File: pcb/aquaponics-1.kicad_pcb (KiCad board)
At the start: 2 copper layers, 67.3 x 63.5 mm, 17 parts, among them J1 5V Power Source, J2 Screw_Terminal_01x02, J3 Water Level Sensor, J4 Rain Sensor, J5 Conn_01x02_Female, M1 Growbed Pump, M2 Overflow Pump, M3 Fish Feeder, Q1 TIP120, Q2 TIP120, Q3 TIP120, U1 Arduino_Nano

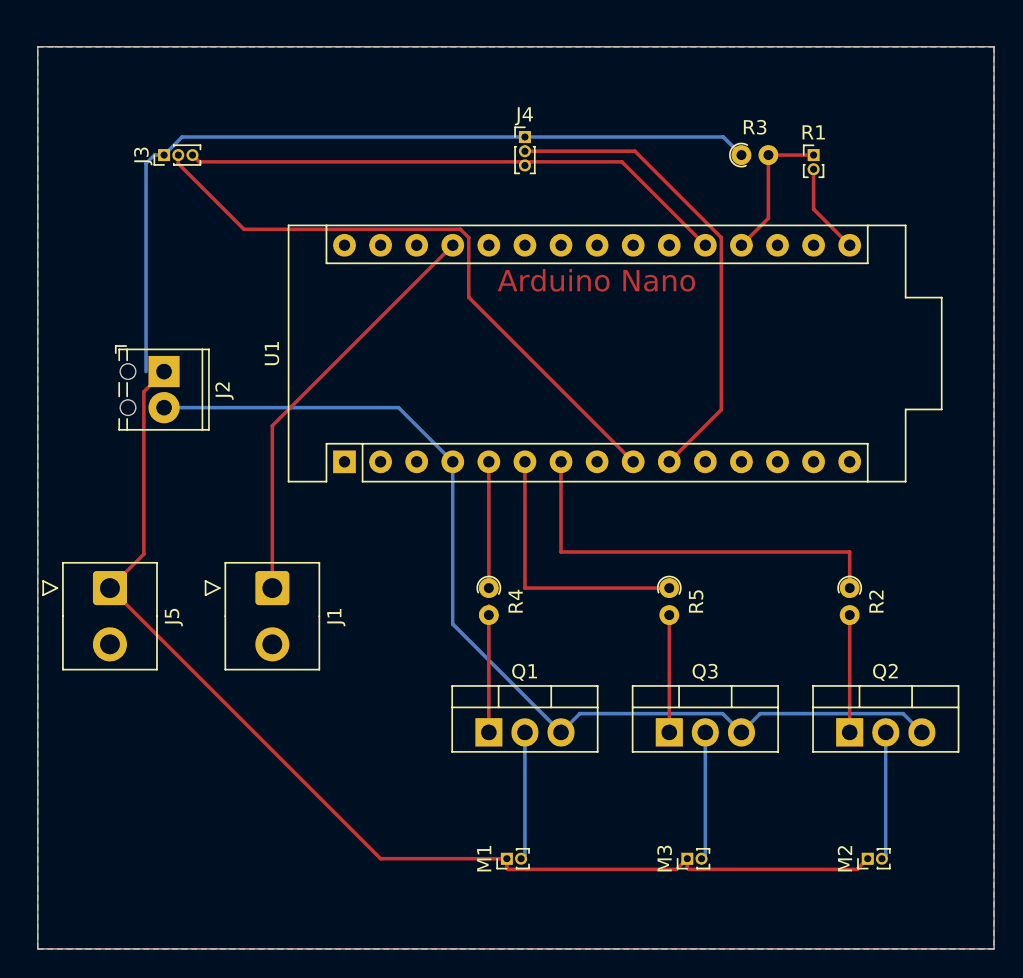
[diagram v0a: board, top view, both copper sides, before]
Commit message: 1st draft
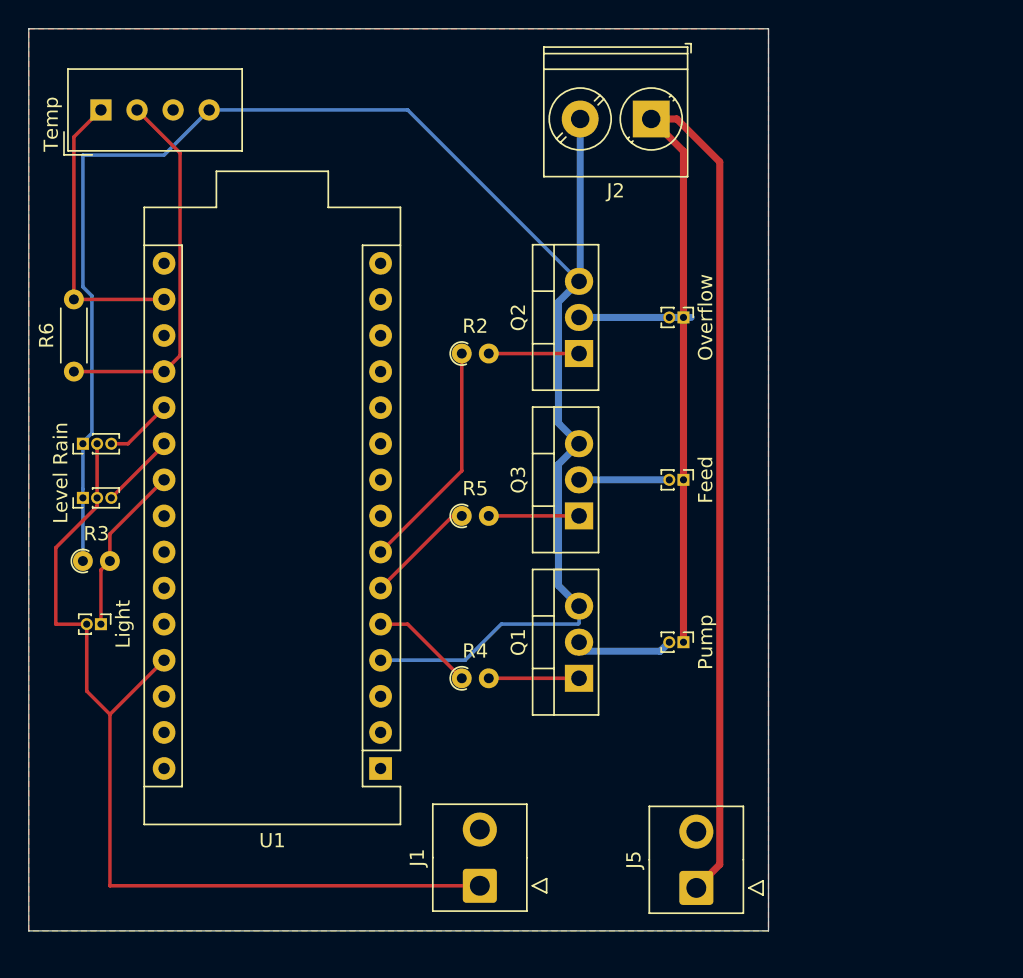
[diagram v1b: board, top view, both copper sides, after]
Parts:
- removed J3: Water Level Sensor, Connector_PinHeader_1.00mm:PinHeader_1x03_P1.00mm_Vertical
- removed J4: Rain Sensor, Connector_PinHeader_1.00mm:PinHeader_1x03_P1.00mm_Vertical
- removed M1: Growbed Pump, Connector_PinHeader_1.00mm:PinHeader_1x02_P1.00mm_Vertical
- removed M2: Overflow Pump, Connector_PinHeader_1.00mm:PinHeader_1x02_P1.00mm_Vertical
- removed M3: Fish Feeder, Connector_PinHeader_1.00mm:PinHeader_1x02_P1.00mm_Vertical
- removed R1: Light Sensor, Connector_PinHeader_1.00mm:PinHeader_1x02_P1.00mm_Vertical
- added Feed: Fish Feeder, Connector_PinHeader_1.00mm:PinHeader_1x02_P1.00mm_Vertical, F.Cu at (64.5, 45.7)
- added Level: Water Level Sensor, Connector_PinHeader_1.00mm:PinHeader_1x03_P1.00mm_Vertical, F.Cu at (22.2, 47.0)
- added Light: Light Sensor, Connector_PinHeader_1.00mm:PinHeader_1x02_P1.00mm_Vertical, F.Cu at (23.5, 55.9)
- added Overflow: Overflow Pump, Connector_PinHeader_1.00mm:PinHeader_1x02_P1.00mm_Vertical, F.Cu at (64.5, 34.3)
- added Pump: Growbed Pump, Connector_PinHeader_1.00mm:PinHeader_1x02_P1.00mm_Vertical, F.Cu at (64.5, 57.1)
- added R6: 10k, Resistor_THT:R_Axial_DIN0204_L3.6mm_D1.6mm_P5.08mm_Horizontal, F.Cu at (21.6, 38.1)
- added Rain: Rain Sensor, Connector_PinHeader_1.00mm:PinHeader_1x03_P1.00mm_Vertical, F.Cu at (22.2, 43.2)
- added Temp: DHT11, Sensor:Aosong_DHT11_5.5x12.0_P2.54mm, F.Cu at (23.5, 19.7)
- J2: footprint TerminalBlock_Phoenix:TerminalBlock_Phoenix_MPT-0,5-2-2.54_1x02_P2.54mm_Horizontal -> TerminalBlock_Phoenix:TerminalBlock_Phoenix_PT-1,5-2-5.0-H_1x02_P5.00mm_Horizontal
- moved R3 54.5 mm to (22.2, 51.4)
- moved J5 46.4 mm to (65.4, 74.4), turned to 90 degrees
- moved J2 38.6 mm to (62.2, 20.3), turned to 180 degrees
- moved Q2 32.8 mm to (57.1, 36.8), turned to 90 degrees
- moved R2 31.9 mm to (48.9, 36.8), turned to 0 degrees
- moved J1 25.5 mm to (50.2, 74.3), turned to 90 degrees
- moved U1 21.7 mm to (43.2, 66.0), turned to 180 degrees
- moved Q3 16.5 mm to (57.1, 48.3), turned to 90 degrees
- moved R5 15.5 mm to (48.9, 48.3), turned to 0 degrees
- moved Q1 7.41 mm to (57.1, 59.7), turned to 90 degrees
- moved R4 6.63 mm to (48.9, 59.7), turned to 0 degrees
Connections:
- net Net-(J1-Pad1) renamed +5V
- J1 pad 2: (no net) -> Net-(J1-Pad2)
- J5 pad 2: (no net) -> Net-(J5-Pad2)
- U1 pad 1: (no net) -> Net-(U1-Pad1)
- U1 pad 11: (no net) -> Net-(U1-Pad11)
- U1 pad 12: (no net) -> Net-(U1-Pad12)
- U1 pad 13: (no net) -> Net-(U1-Pad13)
- U1 pad 14: (no net) -> Net-(U1-Pad14)
- U1 pad 15: (no net) -> Net-(U1-Pad15)
- U1 pad 17: (no net) -> +3V3
- U1 pad 18: (no net) -> Net-(U1-Pad18)
- U1 pad 19: Net-(R1-Pad1) -> Net-(R6-Pad1)
- U1 pad 2: (no net) -> Net-(U1-Pad2)
- U1 pad 22: (no net) -> Net-(R1-Pad1)
- U1 pad 23: (no net) -> Net-(U1-Pad23)
- U1 pad 24: (no net) -> Net-(U1-Pad24)
- U1 pad 25: (no net) -> Net-(U1-Pad25)
- U1 pad 26: (no net) -> Net-(U1-Pad26)
- U1 pad 28: (no net) -> Net-(U1-Pad28)
- U1 pad 29: (no net) -> Net-(U1-Pad29)
- U1 pad 3: (no net) -> Net-(U1-Pad3)
- U1 pad 30: (no net) -> Net-(U1-Pad30)
- U1 pad 8: (no net) -> Net-(U1-Pad8)
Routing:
- net Net-(U1-Pad9): track 43.8 -> 0.00 mm
- net +5V: track 29.4 -> 67.2 mm
- net Net-(J4-Pad3): track 38.7 -> 4.77 mm
- net Net-(U1-Pad10): track 33.6 -> 0.00 mm
- net Net-(R6-Pad1): track 0.00 -> 26.5 mm
- net +3V3: track 0.00 -> 20.5 mm
- net Net-(J2-Pad1): track 80.1 -> 95.6 mm
- net Net-(R2-Pad1): track 29.2 -> 16.3 mm
- net Net-(R5-Pad1): track 19.0 -> 7.82 mm
- net Net-(U1-Pad16): track 6.40 -> 0.00 mm
- net GND: track 129.6 -> 123.3 mm
- net Net-(J3-Pad3): track 0.00 -> 5.35 mm
- net Net-(Q1-Pad1): track 9.52 -> 6.35 mm
- net Net-(M3-Pad2): track 9.00 -> 6.35 mm
- net Net-(Q3-Pad1): track 8.26 -> 6.35 mm
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- removed copper zone on B.Cu, net GND
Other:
- board size 67.3 x 63.5 mm -> 52.1 x 63.5 mm
- board text removed: "Arduino Nano"
